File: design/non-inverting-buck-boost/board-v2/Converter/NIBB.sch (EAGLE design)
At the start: 8 parts

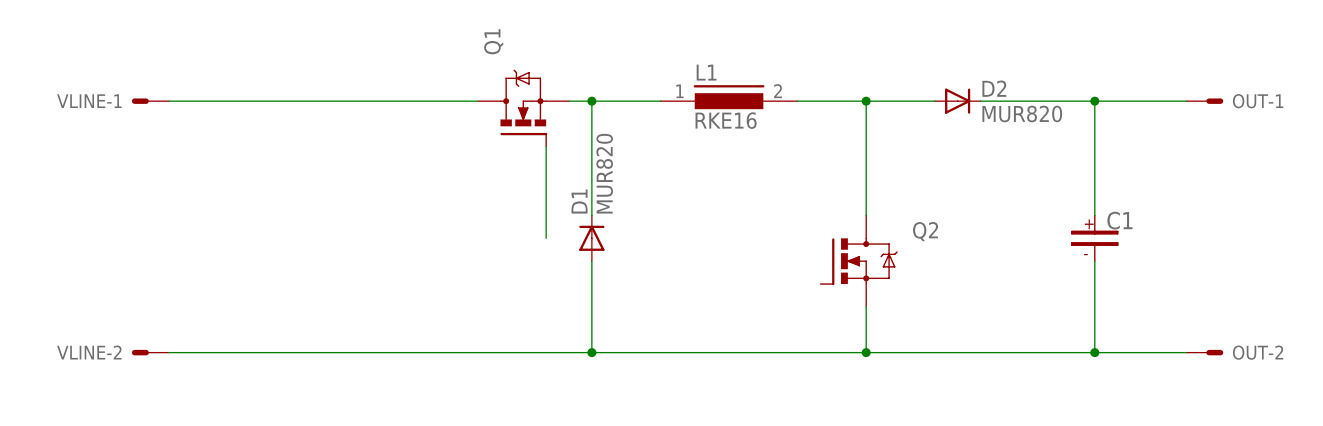
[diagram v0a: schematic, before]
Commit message: finished power board layout
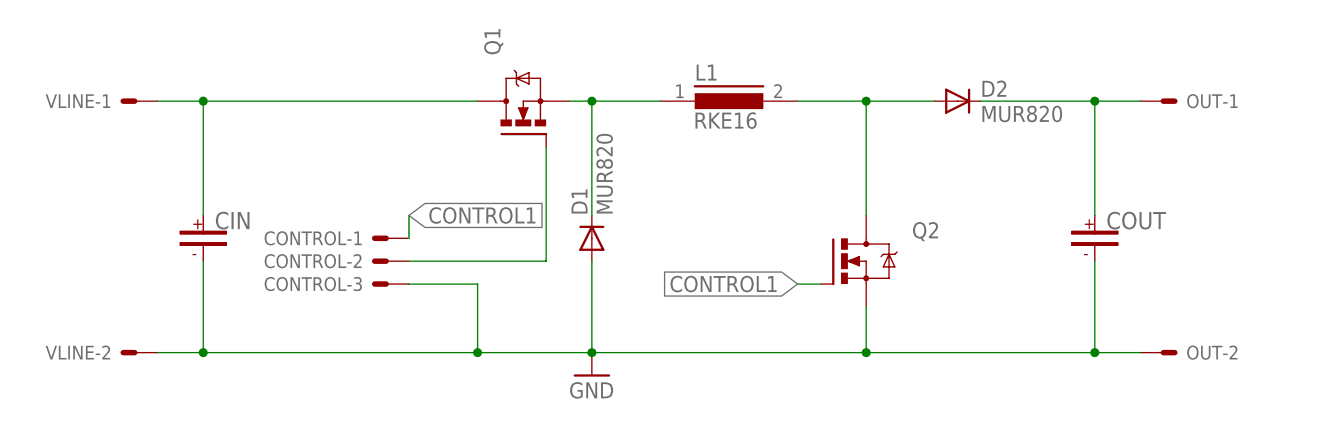
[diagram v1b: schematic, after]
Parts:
- added CIN: (no value), capacitor:CAPP-UF
- added CONTROL: 22-23-2031, con-molex:22-23-2031
- renumbered C1 to COUT
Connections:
- removed net N$4: COUT.-, D1.A, OUT-2.S, Q2.S, VLINE-2.S
- removed net N$5: Q1.G
- new net CONTROL1: CONTROL-1.S, Q2.G
- new net CONTROL2: CONTROL-2.S, Q1.G
- new net GND: CIN.-, CONTROL-3.S, COUT.-, D1.A, OUT-2.S, Q2.S, VLINE-2.S
- net N$3: now also CIN.+
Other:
- moved on the sheet: OUT-1, OUT-2, VLINE-1, VLINE-2
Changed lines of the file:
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@@
 <setting verticaltext="up"/>
 </settings>
-<grid distance="0.1" unitdist="inch" unit="inch" style="lines" multiple="1" display="no" altdistance="0.01" altunitdist="inch" altunit="inch"/>
+<grid distance="0.1" unitdist="inch" unit="inch" style="lines" multiple="1" display="yes" altdistance="0.01" altunitdist="inch" altunit="inch"/>
 <layers>
 <layer number="1" name="Top" color="4" fill="1" visible="no" active="no"/>
@@
 <part name="L1" library="inductors" deviceset="RKE16" device=""/>
 <part name="VLINE" library="con-molex" deviceset="22-23-2021" device="" value=""/>
-<part name="C1" library="capacitor" deviceset="CAPP-U" device="F"/>
+<part name="COUT" library="capacitor" deviceset="CAPP-U" device="F"/>
 <part name="OUT" library="con-molex" deviceset="22-23-2021" device="" value=""/>
 <part name="Q1" library="felippe" deviceset="IRF640" device=""/>
 <part name="Q2" library="felippe" deviceset="IRF640" device=""/>
+<part name="GND1" library="supply1" deviceset="GND" device=""/>
+<part name="CONTROL" library="con-molex" deviceset="22-23-2031" device=""/>
+<part name="CIN" library="capacitor" deviceset="CAPP-U" device="F"/>
 </parts>
 <sheets>
@@
 <instance part="D2" gate="1" x="66.04" y="63.5"/>
 <instance part="L1" gate="1" x="40.64" y="63.5"/>
-<instance part="VLINE" gate="-1" x="-24.13" y="63.5" rot="R180"/>
-<instance part="VLINE" gate="-2" x="-24.13" y="35.56" rot="R180"/>
-<instance part="C1" gate="G$1" x="81.28" y="48.26"/>
-<instance part="OUT" gate="-1" x="93.98" y="63.5" smashed="yes">
-<attribute name="NAME" x="96.52" y="62.738" size="1.524" layer="95"/>
-<attribute name="VALUE" x="98.298" y="59.817" size="1.778" layer="96"/>
+<instance part="VLINE" gate="-1" x="-25.4" y="63.5" rot="R180"/>
+<instance part="VLINE" gate="-2" x="-25.4" y="35.56" rot="R180"/>
+<instance part="COUT" gate="G$1" x="81.28" y="48.26"/>
+<instance part="OUT" gate="-1" x="88.9" y="63.5" smashed="yes">
+<attribute name="NAME" x="91.44" y="62.738" size="1.524" layer="95"/>
+<attribute name="VALUE" x="93.218" y="59.817" size="1.778" layer="96"/>
 </instance>
-<instance part="OUT" gate="-2" x="93.98" y="35.56"/>
+<instance part="OUT" gate="-2" x="88.9" y="35.56"/>
 <instance part="Q1" gate="G$1" x="17.78" y="60.96" rot="R90"/>
 <instance part="Q2" gate="G$1" x="53.34" y="45.72"/>
+<instance part="GND1" gate="1" x="25.4" y="33.02"/>
+<instance part="CONTROL" gate="-1" x="2.54" y="48.26" smashed="yes" rot="R180">
+<attribute name="NAME" x="0" y="49.022" size="1.524" layer="95" rot="R180"/>
+</instance>
+<instance part="CONTROL" gate="-2" x="2.54" y="45.72" rot="R180"/>
+<instance part="CONTROL" gate="-3" x="2.54" y="43.18" rot="R180"/>
+<instance part="CIN" gate="G$1" x="-17.78" y="48.26"/>
 </instances>
 <busses>
@@
 </segment>
 </net>
-<net name="N$4" class="0">
+<net name="N$3" class="0">
+<segment>
+<pinref part="VLINE" gate="-1" pin="S"/>
+<wire x1="-22.86" y1="63.5" x2="-17.78" y2="63.5" width="0.1524" layer="91"/>
+<pinref part="Q1" gate="G$1" pin="D"/>
+<pinref part="CIN" gate="G$1" pin="+"/>
+<wire x1="-17.78" y1="63.5" x2="12.7" y2="63.5" width="0.1524" layer="91"/>
+<wire x1="-17.78" y1="50.8" x2="-17.78" y2="63.5" width="0.1524" layer="91"/>
+<junction x="-17.78" y="63.5"/>
+</segment>
+</net>
+<net name="CONTROL1" class="0">
+<segment>
+<pinref part="Q2" gate="G$1" pin="G"/>
+<wire x1="50.8" y1="43.18" x2="48.26" y2="43.18" width="0.1524" layer="91"/>
+<label x="48.26" y="43.18" size="1.778" layer="95" rot="R180" xref="yes"/>
+</segment>
+<segment>
+<pinref part="CONTROL" gate="-1" pin="S"/>
+<wire x1="5.08" y1="48.26" x2="5.08" y2="50.8" width="0.1524" layer="91"/>
+<label x="5.08" y="50.8" size="1.778" layer="95" xref="yes"/>
+</segment>
+</net>
+<net name="N$7" class="0">
+<segment>
+<pinref part="D2" gate="1" pin="C"/>
+<wire x1="68.58" y1="63.5" x2="81.28" y2="63.5" width="0.1524" layer="91"/>
+<wire x1="81.28" y1="63.5" x2="81.28" y2="50.8" width="0.1524" layer="91"/>
+<pinref part="COUT" gate="G$1" pin="+"/>
+<pinref part="OUT" gate="-1" pin="S"/>
+<wire x1="86.36" y1="63.5" x2="81.28" y2="63.5" width="0.1524" layer="91"/>
+<junction x="81.28" y="63.5"/>
+</segment>
+</net>
+<net name="N$1" class="0">
+<segment>
+<pinref part="L1" gate="1" pin="1"/>
+<wire x1="22.86" y1="63.5" x2="25.4" y2="63.5" width="0.1524" layer="91"/>
+<pinref part="D1" gate="1" pin="C"/>
+<wire x1="25.4" y1="63.5" x2="33.02" y2="63.5" width="0.1524" layer="91"/>
+<wire x1="25.4" y1="50.8" x2="25.4" y2="63.5" width="0.1524" layer="91"/>
+<junction x="25.4" y="63.5"/>
+<pinref part="Q1" gate="G$1" pin="S"/>
+</segment>
+</net>
+<net name="GND" class="0">
 <segment>
 <wire x1="55.88" y1="40.64" x2="55.88" y2="35.56" width="0.1524" layer="91"/>
 <pinref part="VLINE" gate="-2" pin="S"/>
-<wire x1="-21.59" y1="35.56" x2="25.4" y2="35.56" width="0.1524" layer="91"/>
-<pinref part="C1" gate="G$1" pin="-"/>
+<wire x1="-22.86" y1="35.56" x2="-17.78" y2="35.56" width="0.1524" layer="91"/>
+<pinref part="COUT" gate="G$1" pin="-"/>
+<wire x1="-17.78" y1="35.56" x2="12.7" y2="35.56" width="0.1524" layer="91"/>
+<wire x1="12.7" y1="35.56" x2="25.4" y2="35.56" width="0.1524" layer="91"/>
 <wire x1="25.4" y1="35.56" x2="55.88" y2="35.56" width="0.1524" layer="91"/>
 <wire x1="81.28" y1="45.72" x2="81.28" y2="35.56" width="0.1524" layer="91"/>
@@
 <junction x="25.4" y="35.56"/>
 <pinref part="OUT" gate="-2" pin="S"/>
-<wire x1="91.44" y1="35.56" x2="81.28" y2="35.56" width="0.1524" layer="91"/>
+<wire x1="86.36" y1="35.56" x2="81.28" y2="35.56" width="0.1524" layer="91"/>
 <junction x="81.28" y="35.56"/>
 <pinref part="Q2" gate="G$1" pin="S"/>
-</segment>
-</net>
-<net name="N$3" class="0">
-<segment>
-<pinref part="VLINE" gate="-1" pin="S"/>
-<wire x1="-21.59" y1="63.5" x2="12.7" y2="63.5" width="0.1524" layer="91"/>
-<pinref part="Q1" gate="G$1" pin="D"/>
-</segment>
-</net>
-<net name="N$5" class="0">
-<segment>
-<wire x1="20.32" y1="48.26" x2="20.32" y2="58.42" width="0.1524" layer="91"/>
+<pinref part="GND1" gate="1" pin="GND"/>
+<pinref part="CONTROL" gate="-3" pin="S"/>
+<wire x1="5.08" y1="43.18" x2="12.7" y2="43.18" width="0.1524" layer="91"/>
+<wire x1="12.7" y1="43.18" x2="12.7" y2="35.56" width="0.1524" layer="91"/>
+<junction x="12.7" y="35.56"/>
+<pinref part="CIN" gate="G$1" pin="-"/>
+<wire x1="-17.78" y1="45.72" x2="-17.78" y2="35.56" width="0.1524" layer="91"/>
+<junction x="-17.78" y="35.56"/>
+</segment>
+</net>
+<net name="CONTROL2" class="0">
+<segment>
+<pinref part="CONTROL" gate="-2" pin="S"/>
+<wire x1="5.08" y1="45.72" x2="20.32" y2="45.72" width="0.1524" layer="91"/>
 <pinref part="Q1" gate="G$1" pin="G"/>
-</segment>
-</net>
-<net name="N$7" class="0">
-<segment>
-<pinref part="D2" gate="1" pin="C"/>
-<wire x1="68.58" y1="63.5" x2="81.28" y2="63.5" width="0.1524" layer="91"/>
-<wire x1="81.28" y1="63.5" x2="81.28" y2="50.8" width="0.1524" layer="91"/>
-<pinref part="C1" gate="G$1" pin="+"/>
-<pinref part="OUT" gate="-1" pin="S"/>
-<wire x1="91.44" y1="63.5" x2="81.28" y2="63.5" width="0.1524" layer="91"/>
-<junction x="81.28" y="63.5"/>
-</segment>
-</net>
-<net name="N$1" class="0">
-<segment>
-<pinref part="L1" gate="1" pin="1"/>
-<wire x1="22.86" y1="63.5" x2="25.4" y2="63.5" width="0.1524" layer="91"/>
-<pinref part="D1" gate="1" pin="C"/>
-<wire x1="25.4" y1="63.5" x2="33.02" y2="63.5" width="0.1524" layer="91"/>
-<wire x1="25.4" y1="50.8" x2="25.4" y2="63.5" width="0.1524" layer="91"/>
-<junction x="25.4" y="63.5"/>
-<pinref part="Q1" gate="G$1" pin="S"/>
-</segment>
-</net>
+<wire x1="20.32" y1="45.72" x2="20.32" y2="58.42" width="0.1524" layer="91"/>
+</segment>
+</net>
